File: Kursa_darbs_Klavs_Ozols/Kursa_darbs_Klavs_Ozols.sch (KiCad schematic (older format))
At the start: 31 parts, among them J1 Barosana, J11 Conn_01x01, J12 Conn_01x01, J13 Conn_01x01, J14 Conn_01x01, J15 Conn_01x01, J16 Conn_01x01, J17 Conn_01x01, J18 Conn_01x01, J19 Conn_01x01, J2 Audio-Jack-3, J20 Conn_01x01, J3 Conn_01x01, J34 Conn_01x01, J35 Conn_01x01, J36 Conn_01x01, J39 Conn_01x01, J4 Conn_01x01, J40 Conn_01x01, J41 Conn_01x01, J42 Conn_01x01, J43 Conn_01x01, J44 Conn_01x01, J45 Conn_01x01, J46 Conn_01x01, J5 Conn_01x01, J52 Conn_01x01, J6 Conn_01x01, J7 Conn_01x01, J8 Conn_01x01, J9 Conn_01x01

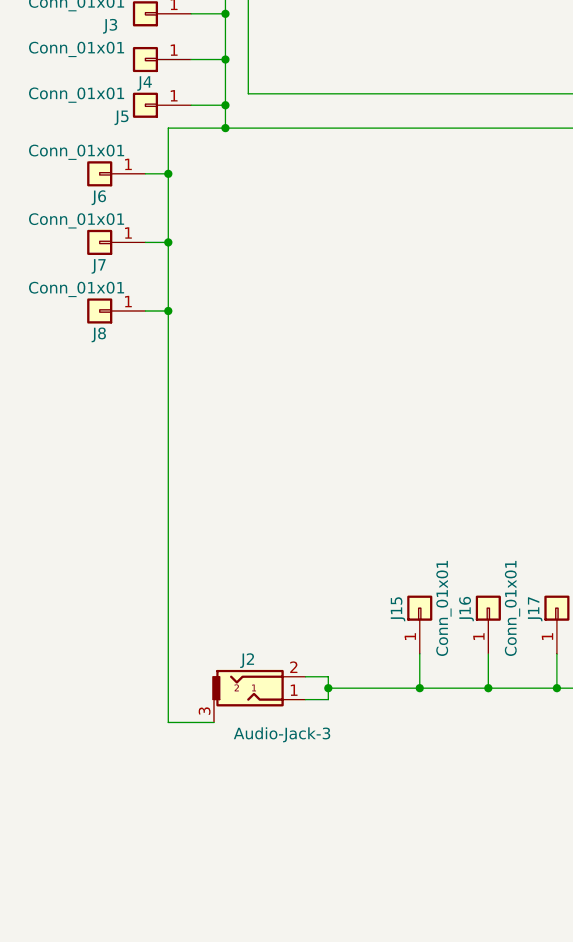
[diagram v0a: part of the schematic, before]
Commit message: 1. Prototipa finaala versija
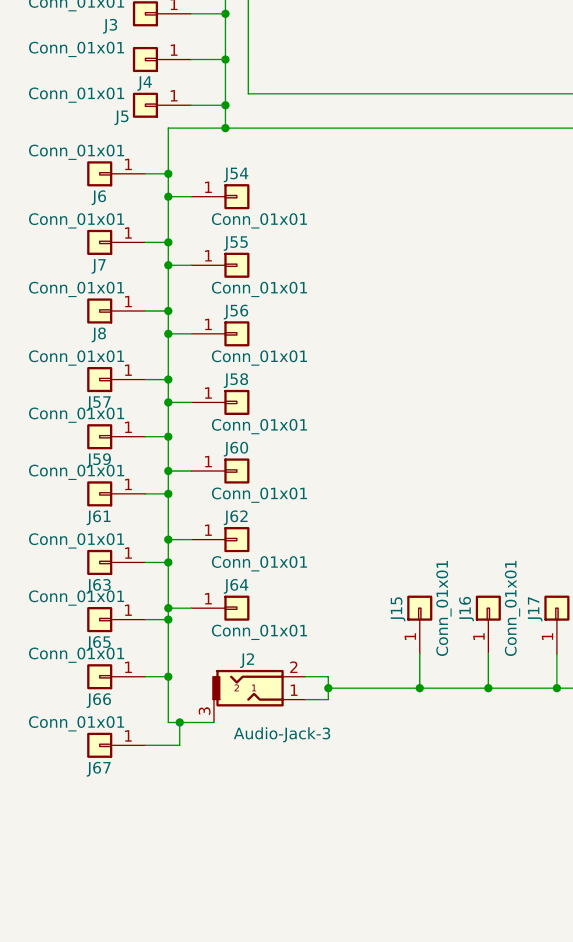
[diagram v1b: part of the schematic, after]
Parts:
- added J54, J55, J56, J57, J58, J59, J60, J61, J62, J63, J64, J65, J66, J67: Conn_01x01, Mounting_Holes:MountingHole_3.2mm_M3_Pad_Via, symbol Conn_01x01
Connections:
- net GND: now also J54.1 (Pin_1), J55.1 (Pin_1), J56.1 (Pin_1), J57.1 (Pin_1), J58.1 (Pin_1), J59.1 (Pin_1), J60.1 (Pin_1), J61.1 (Pin_1), J62.1 (Pin_1), J63.1 (Pin_1), J64.1 (Pin_1), J65.1 (Pin_1), J66.1 (Pin_1), J67.1 (Pin_1)
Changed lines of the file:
@@
 	10150 700  10150 950
 Connection ~ 10150 950
+$Comp
+L Conn_01x01 J57
+U 1 1 5B255C18
+P 850 3750
+F 0 "J57" H 850 3850 50  0000 C CNN
+F 1 "Conn_01x01" H 950 3650 50  0000 C CNN
+F 2 "Mounting_Holes:MountingHole_3.2mm_M3_Pad_Via" H 850 3750 50  0001 C CNN
+F 3 "" H 850 3750 50  0001 C CNN
+	1    850  3750
+	-1   0    0    1
+$EndComp
+$Comp
+L Conn_01x01 J59
+U 1 1 5B256229
+P 850 4000
+F 0 "J59" H 850 4100 50  0000 C CNN
+F 1 "Conn_01x01" H 950 3900 50  0000 C CNN
+F 2 "Mounting_Holes:MountingHole_3.2mm_M3_Pad_Via" H 850 4000 50  0001 C CNN
+F 3 "" H 850 4000 50  0001 C CNN
+	1    850  4000
+	-1   0    0    1
+$EndComp
+$Comp
+L Conn_01x01 J61
+U 1 1 5B2564BA
+P 850 4250
+F 0 "J61" H 850 4350 50  0000 C CNN
+F 1 "Conn_01x01" H 950 4150 50  0000 C CNN
+F 2 "Mounting_Holes:MountingHole_3.2mm_M3_Pad_Via" H 850 4250 50  0001 C CNN
+F 3 "" H 850 4250 50  0001 C CNN
+	1    850  4250
+	-1   0    0    1
+$EndComp
+$Comp
+L Conn_01x01 J63
+U 1 1 5B2569A6
+P 850 4550
+F 0 "J63" H 850 4650 50  0000 C CNN
+F 1 "Conn_01x01" H 950 4450 50  0000 C CNN
+F 2 "Mounting_Holes:MountingHole_3.2mm_M3_Pad_Via" H 850 4550 50  0001 C CNN
+F 3 "" H 850 4550 50  0001 C CNN
+	1    850  4550
+	-1   0    0    1
+$EndComp
+$Comp
+L Conn_01x01 J65
+U 1 1 5B256C3D
+P 850 4800
+F 0 "J65" H 850 4900 50  0000 C CNN
+F 1 "Conn_01x01" H 950 4700 50  0000 C CNN
+F 2 "Mounting_Holes:MountingHole_3.2mm_M3_Pad_Via" H 850 4800 50  0001 C CNN
+F 3 "" H 850 4800 50  0001 C CNN
+	1    850  4800
+	-1   0    0    1
+$EndComp
+$Comp
+L Conn_01x01 J66
+U 1 1 5B256ED9
+P 850 5050
+F 0 "J66" H 850 5150 50  0000 C CNN
+F 1 "Conn_01x01" H 950 4950 50  0000 C CNN
+F 2 "Mounting_Holes:MountingHole_3.2mm_M3_Pad_Via" H 850 5050 50  0001 C CNN
+F 3 "" H 850 5050 50  0001 C CNN
+	1    850  5050
+	-1   0    0    1
+$EndComp
+$Comp
+L Conn_01x01 J67
+U 1 1 5B257178
+P 850 5350
+F 0 "J67" H 850 5450 50  0000 C CNN
+F 1 "Conn_01x01" H 950 5250 50  0000 C CNN
+F 2 "Mounting_Holes:MountingHole_3.2mm_M3_Pad_Via" H 850 5350 50  0001 C CNN
+F 3 "" H 850 5350 50  0001 C CNN
+	1    850  5350
+	-1   0    0    1
+$EndComp
+$Comp
+L Conn_01x01 J54
+U 1 1 5B257549
+P 1450 2950
+F 0 "J54" H 1450 3050 50  0000 C CNN
+F 1 "Conn_01x01" H 1550 2850 50  0000 C CNN
+F 2 "Mounting_Holes:MountingHole_3.2mm_M3_Pad_Via" H 1450 2950 50  0001 C CNN
+F 3 "" H 1450 2950 50  0001 C CNN
+	1    1450 2950
+	1    0    0    -1
+$EndComp
+$Comp
+L Conn_01x01 J55
+U 1 1 5B257A84
+P 1450 3250
+F 0 "J55" H 1450 3350 50  0000 C CNN
+F 1 "Conn_01x01" H 1550 3150 50  0000 C CNN
+F 2 "Mounting_Holes:MountingHole_3.2mm_M3_Pad_Via" H 1450 3250 50  0001 C CNN
+F 3 "" H 1450 3250 50  0001 C CNN
+	1    1450 3250
+	1    0    0    -1
+$EndComp
+$Comp
+L Conn_01x01 J56
+U 1 1 5B257D34
+P 1450 3550
+F 0 "J56" H 1450 3650 50  0000 C CNN
+F 1 "Conn_01x01" H 1550 3450 50  0000 C CNN
+F 2 "Mounting_Holes:MountingHole_3.2mm_M3_Pad_Via" H 1450 3550 50  0001 C CNN
+F 3 "" H 1450 3550 50  0001 C CNN
+	1    1450 3550
+	1    0    0    -1
+$EndComp
+$Comp
+L Conn_01x01 J58
+U 1 1 5B257FDD
+P 1450 3850
+F 0 "J58" H 1450 3950 50  0000 C CNN
+F 1 "Conn_01x01" H 1550 3750 50  0000 C CNN
+F 2 "Mounting_Holes:MountingHole_3.2mm_M3_Pad_Via" H 1450 3850 50  0001 C CNN
+F 3 "" H 1450 3850 50  0001 C CNN
+	1    1450 3850
+	1    0    0    -1
+$EndComp
+$Comp
+L Conn_01x01 J60
+U 1 1 5B2589FD
+P 1450 4150
+F 0 "J60" H 1450 4250 50  0000 C CNN
+F 1 "Conn_01x01" H 1550 4050 50  0000 C CNN
+F 2 "Mounting_Holes:MountingHole_3.2mm_M3_Pad_Via" H 1450 4150 50  0001 C CNN
+F 3 "" H 1450 4150 50  0001 C CNN
+	1    1450 4150
+	1    0    0    -1
+$EndComp
+$Comp
+L Conn_01x01 J62
+U 1 1 5B258CBA
+P 1450 4450
+F 0 "J62" H 1450 4550 50  0000 C CNN
+F 1 "Conn_01x01" H 1550 4350 50  0000 C CNN
+F 2 "Mounting_Holes:MountingHole_3.2mm_M3_Pad_Via" H 1450 4450 50  0001 C CNN
+F 3 "" H 1450 4450 50  0001 C CNN
+	1    1450 4450
+	1    0    0    -1
+$EndComp
+$Comp
+L Conn_01x01 J64
+U 1 1 5B258F6C
+P 1450 4750
+F 0 "J64" H 1450 4850 50  0000 C CNN
+F 1 "Conn_01x01" H 1550 4650 50  0000 C CNN
+F 2 "Mounting_Holes:MountingHole_3.2mm_M3_Pad_Via" H 1450 4750 50  0001 C CNN
+F 3 "" H 1450 4750 50  0001 C CNN
+	1    1450 4750
+	1    0    0    -1
+$EndComp
+Wire Wire Line
+	1250 2950 1150 2950
+Connection ~ 1150 2950
+Wire Wire Line
+	1250 3250 1150 3250
+Connection ~ 1150 3250
+Wire Wire Line
+	1250 3550 1150 3550
+Connection ~ 1150 3550
+Wire Wire Line
+	1050 3750 1150 3750
+Connection ~ 1150 3750
+Wire Wire Line
+	1250 3850 1150 3850
+Connection ~ 1150 3850
+Wire Wire Line
+	1050 4000 1150 4000
+Connection ~ 1150 4000
+Wire Wire Line
+	1250 4150 1150 4150
+Connection ~ 1150 4150
+Wire Wire Line
+	1050 4250 1150 4250
+Connection ~ 1150 4250
+Wire Wire Line
+	1250 4450 1150 4450
+Connection ~ 1150 4450
+Wire Wire Line
+	1050 4550 1150 4550
+Connection ~ 1150 4550
+Wire Wire Line
+	1250 4750 1150 4750
+Connection ~ 1150 4750
+Wire Wire Line
+	1050 4800 1150 4800
+Connection ~ 1150 4800
+Wire Wire Line
+	1050 5050 1150 5050
+Connection ~ 1150 5050
+Wire Wire Line
+	1050 5350 1200 5350
+Wire Wire Line
+	1200 5350 1200 5250
+Connection ~ 1200 5250
 $EndSCHEMATC
